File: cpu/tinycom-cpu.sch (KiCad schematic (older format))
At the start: 4 parts, among them P1 CONN_02X08, P2 CONN_02X08, U1 OLIMEX_IC_A13, U2 H5TQG63BFR/FBGA96

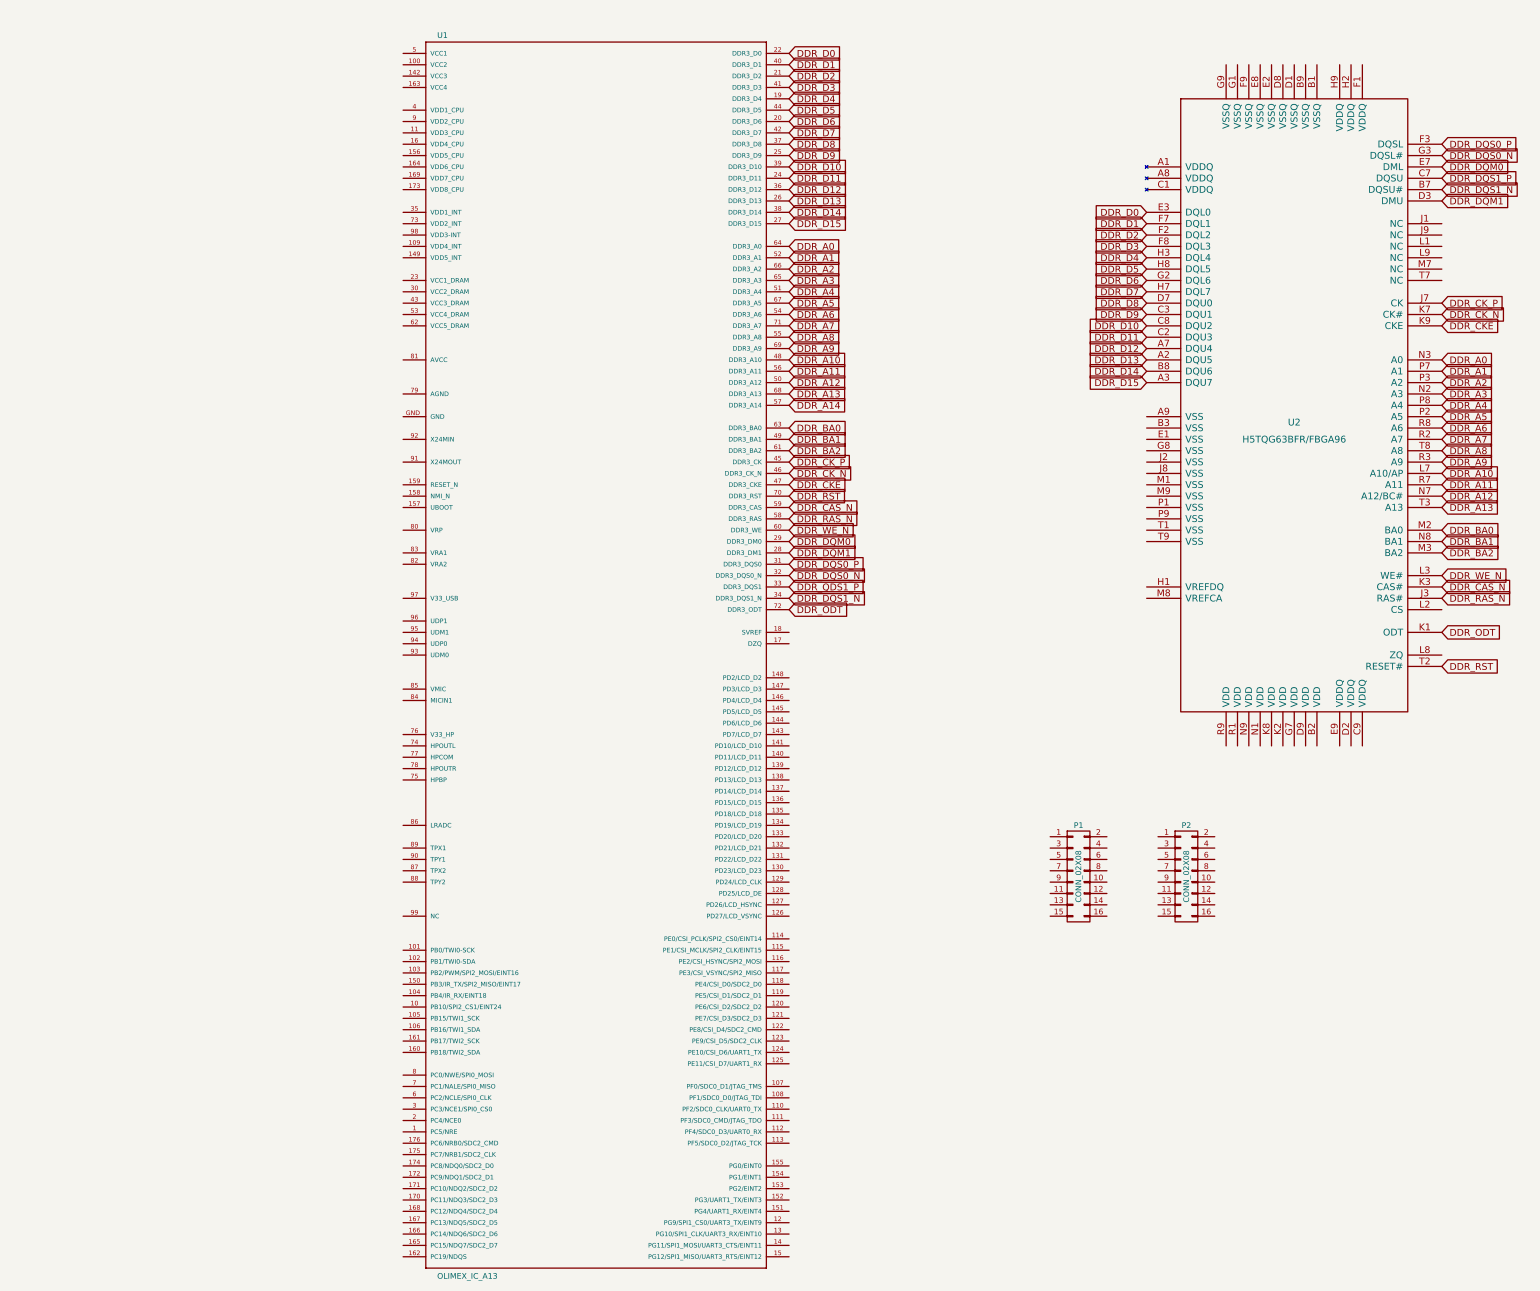
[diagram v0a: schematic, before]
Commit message: add routes
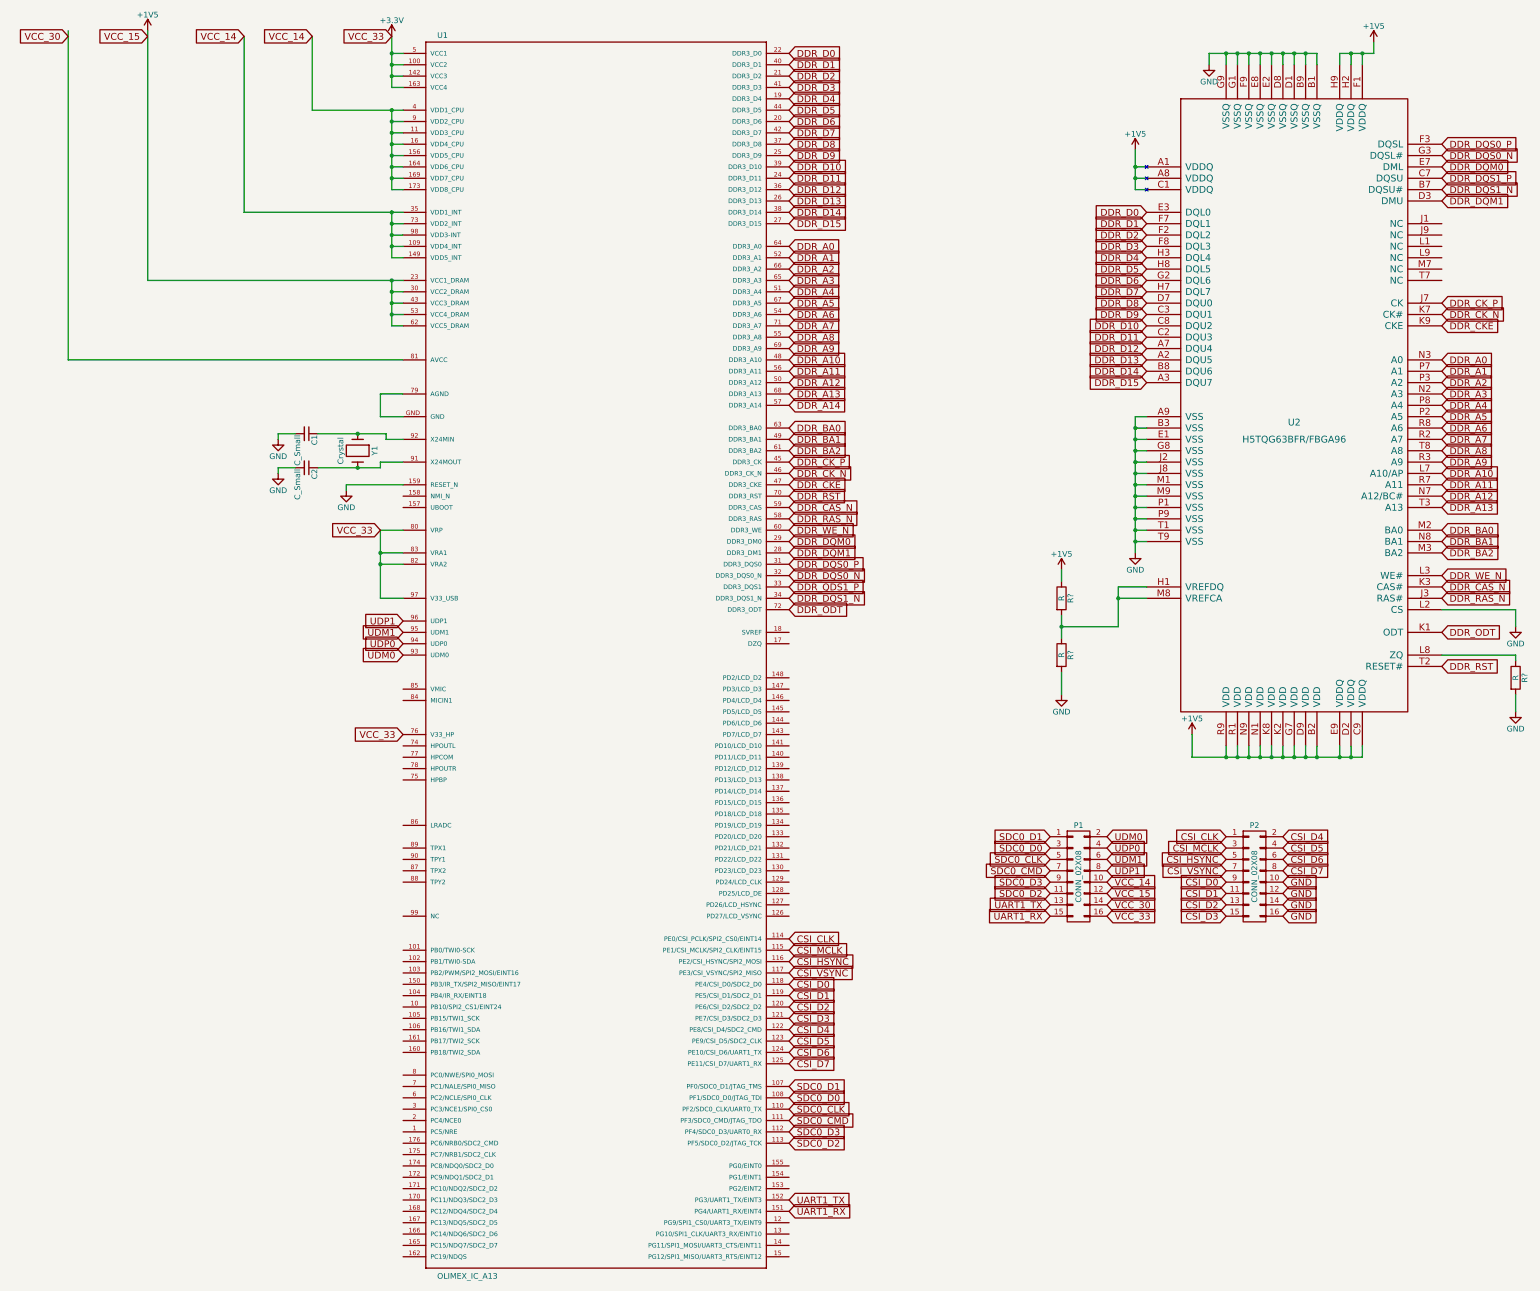
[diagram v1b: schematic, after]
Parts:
- added C1, C2: C_Small, Capacitors_SMD:C_0402, symbol C_Small
- added R? (x3): R, symbol R
- added Y1: Crystal, Crystals:crystal_FA238-TSX3225, symbol Crystal
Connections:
- net +1V5: now reaches U2.A1 (VDDQ)
- net +1V5: now also P1.12 (P12), U1.23 (VCC1_DRAM), U1.30 (VCC2_DRAM), U1.43 (VCC3_DRAM), U1.53 (VCC4_DRAM), U1.62 (VCC5_DRAM), U2.A8 (VDDQ), U2.B2 (VDD), U2.C1 (VDDQ), U2.C9 (VDDQ), U2.D2 (VDDQ), U2.D9 (VDD), U2.E9 (VDDQ), U2.F1 (VDDQ), U2.G7 (VDD), U2.H2 (VDDQ), U2.H9 (VDDQ), U2.K2 (VDD), U2.K8 (VDD), U2.N1 (VDD), U2.N9 (VDD), U2.R1 (VDD), U2.R9 (VDD), R?.1
- net GND: now reaches U2.A9 (VSS)
- net GND: now also P2.10 (P10), P2.12 (P12), P2.14 (P14), P2.16 (P16), U1.159 (RESET_N), U2.B1 (VSSQ), U2.B3 (VSS), U2.B9 (VSSQ), U2.D1 (VSSQ), U2.D8 (VSSQ), U2.E1 (VSS), U2.E2 (VSSQ), U2.E8 (VSSQ), U2.F9 (VSSQ), U2.G1 (VSSQ), U2.G8 (VSS), U2.G9 (VSSQ), U2.J2 (VSS), U2.J8 (VSS), U2.L2 (CS), U2.M1 (VSS), U2.M9 (VSS), U2.P1 (VSS), U2.P9 (VSS), U2.T1 (VSS), U2.T9 (VSS), C1.2, C2.2, R?.2, R?.2
- net at U2.H1 (VREFDQ): now also U2.M8 (VREFCA), R?.1, R?.2
- net at U2.L8 (ZQ): now also R?.1
- net +3V3: now reaches U1.100 (VCC2)
- net +3V3: now also P1.16 (P16), U1.142 (VCC3), U1.163 (VCC4), U1.5 (VCC1), U1.76 (V33_HP), U1.80 (VRP), U1.82 (VRA2), U1.83 (VRA1), U1.97 (V33_USB)
- net SDC0_D1: now reaches U1.107 (PF0/SDC0_D1/JTAG_TMS)
- net SDC0_D1: now also P1.1 (P1)
- net SDC0_D0: now reaches U1.108 (PF1/SDC0_D0/JTAG_TDI)
- net SDC0_D0: now also P1.3 (P3)
- net VCC_14: now reaches U1.109 (VDD4_INT)
- net VCC_14: now also P1.10 (P10), U1.11 (VDD3_CPU), U1.149 (VDD5_INT), U1.156 (VDD5_CPU), U1.16 (VDD4_CPU), U1.164 (VDD6_CPU), U1.169 (VDD7_CPU), U1.173 (VDD8_CPU), U1.35 (VDD1_INT), U1.4 (VDD1_CPU), U1.73 (VDD2_INT), U1.9 (VDD2_CPU), U1.98 (VDD3-INT)
- net SDC0_CLK: now reaches U1.110 (PF2/SDC0_CLK/UART0_TX)
- net SDC0_CLK: now also P1.5 (P5)
- net SDC0_CMD: now reaches U1.111 (PF3/SDC0_CMD/JTAG_TDO)
- net SDC0_CMD: now also P1.7 (P7)
- net SDC0_D3: now reaches U1.112 (PF4/SDC0_D3/UART0_RX)
- net SDC0_D3: now also P1.9 (P9)
- net SDC0_D2: now reaches U1.113 (PF5/SDC0_D2/JTAG_TCK)
- net SDC0_D2: now also P1.11 (P11)
- net CSI_CLK: now reaches U1.114 (PE0/CSI_PCLK/SPI2_CS0/EINT14)
- net CSI_CLK: now also P2.1 (P1)
- net CSI_MCLK: now reaches U1.115 (PE1/CSI_MCLK/SPI2_CLK/EINT15)
- net CSI_MCLK: now also P2.3 (P3)
- net CSI_HSYNC: now reaches U1.116 (PE2/CSI_HSYNC/SPI2_MOSI)
- net CSI_HSYNC: now also P2.5 (P5)
- net CSI_VSYNC: now reaches U1.117 (PE3/CSI_VSYNC/SPI2_MISO)
- net CSI_VSYNC: now also P2.7 (P7)
- net CSI_D0: now reaches U1.118 (PE4/CSI_D0/SDC2_D0)
- net CSI_D0: now also P2.9 (P9)
- net CSI_D1: now reaches U1.119 (PE5/CSI_D1/SDC2_D1)
- net CSI_D1: now also P2.11 (P11)
- net CSI_D2: now reaches U1.120 (PE6/CSI_D2/SDC2_D2)
- net CSI_D2: now also P2.13 (P13)
- net CSI_D3: now reaches U1.121 (PE7/CSI_D3/SDC2_D3)
- net CSI_D3: now also P2.15 (P15)
- net CSI_D4: now reaches U1.122 (PE8/CSI_D4/SDC2_CMD)
- net CSI_D4: now also P2.2 (P2)
- net CSI_D5: now reaches U1.123 (PE9/CSI_D5/SDC2_CLK)
- net CSI_D5: now also P2.4 (P4)
- net CSI_D6: now reaches U1.124 (PE10/CSI_D6/UART1_TX)
- net CSI_D6: now also P2.6 (P6)
- net CSI_D7: now reaches U1.125 (PE11/CSI_D7/UART1_RX)
- net CSI_D7: now also P2.8 (P8)
- net UART1_RX: now reaches U1.151 (PG4/UART1_RX/EINT4)
- net UART1_RX: now also P1.15 (P15)
- net UART1_TX: now reaches U1.152 (PG3/UART1_TX/EINT3)
- net UART1_TX: now also P1.13 (P13)
- net at U1.79 (AGND): now also U1.GND_ (GND)
- net VCC_30: now reaches U1.81 (AVCC)
- net VCC_30: now also P1.14 (P14)
- net at U1.91 (X24MOUT): now also C2.1, Y1.2
- net at U1.92 (X24MIN): now also C1.1, Y1.1
- net UDM0: now reaches U1.93 (UDM0)
- net UDM0: now also P1.2 (P2)
- net UDP0: now reaches U1.94 (UDP0)
- net UDP0: now also P1.4 (P4)
- net UDM1: now reaches U1.95 (UDM1)
- net UDM1: now also P1.6 (P6)
- net UDP1: now reaches U1.96 (UDP1)
- net UDP1: now also P1.8 (P8)
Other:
- moved on the sheet: P2
